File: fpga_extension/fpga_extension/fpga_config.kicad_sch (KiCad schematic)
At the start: 19 parts, among them U6 LFE5UM-85F-6BG381x

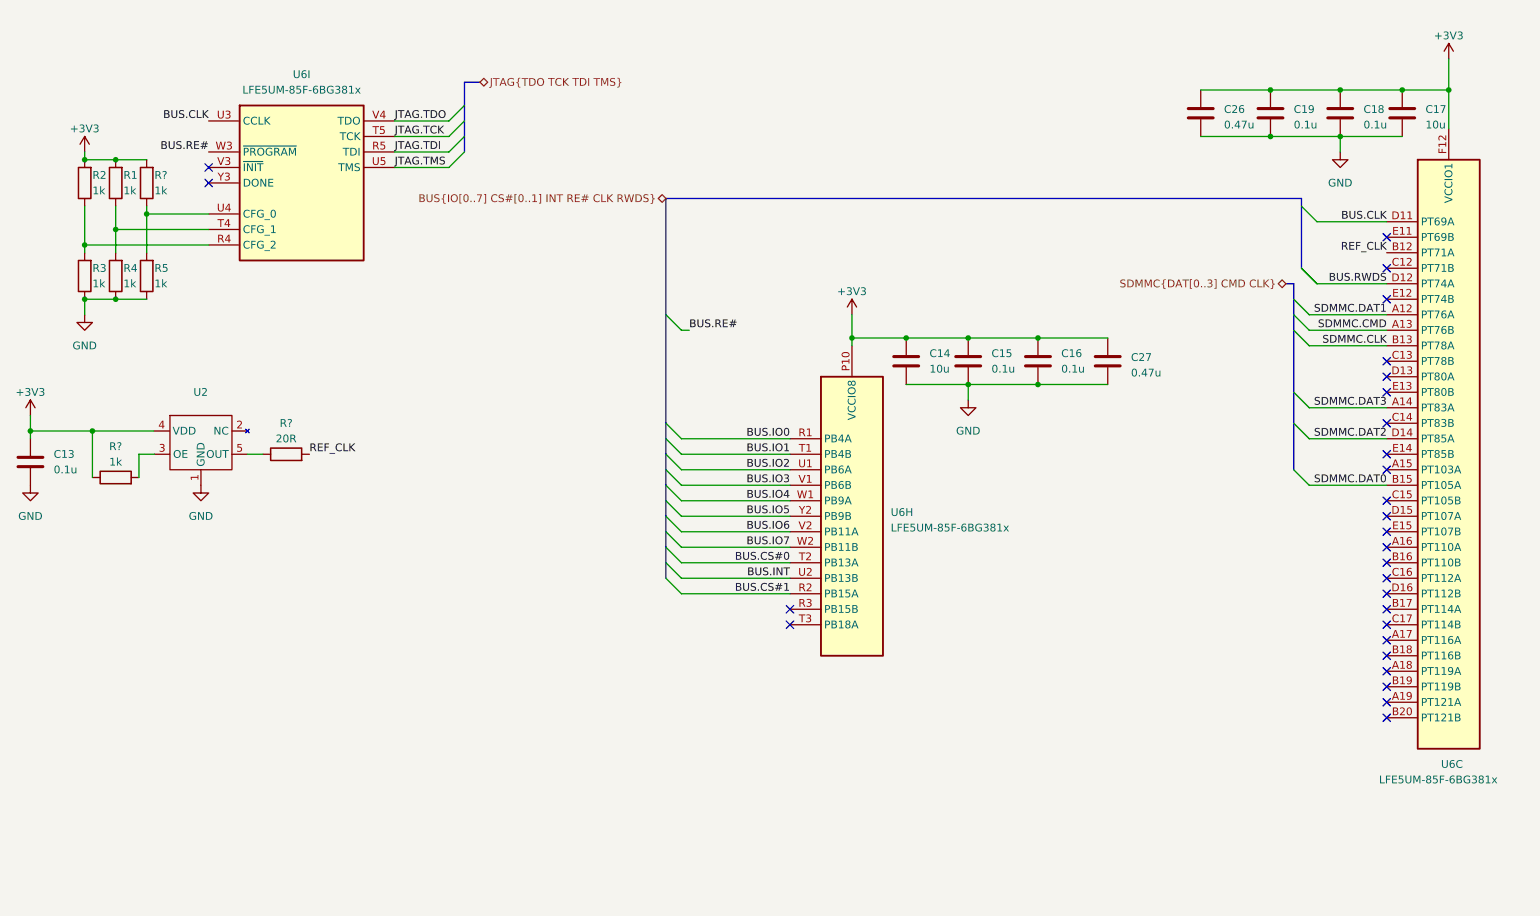
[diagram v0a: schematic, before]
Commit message: prepared first versions of PCBs
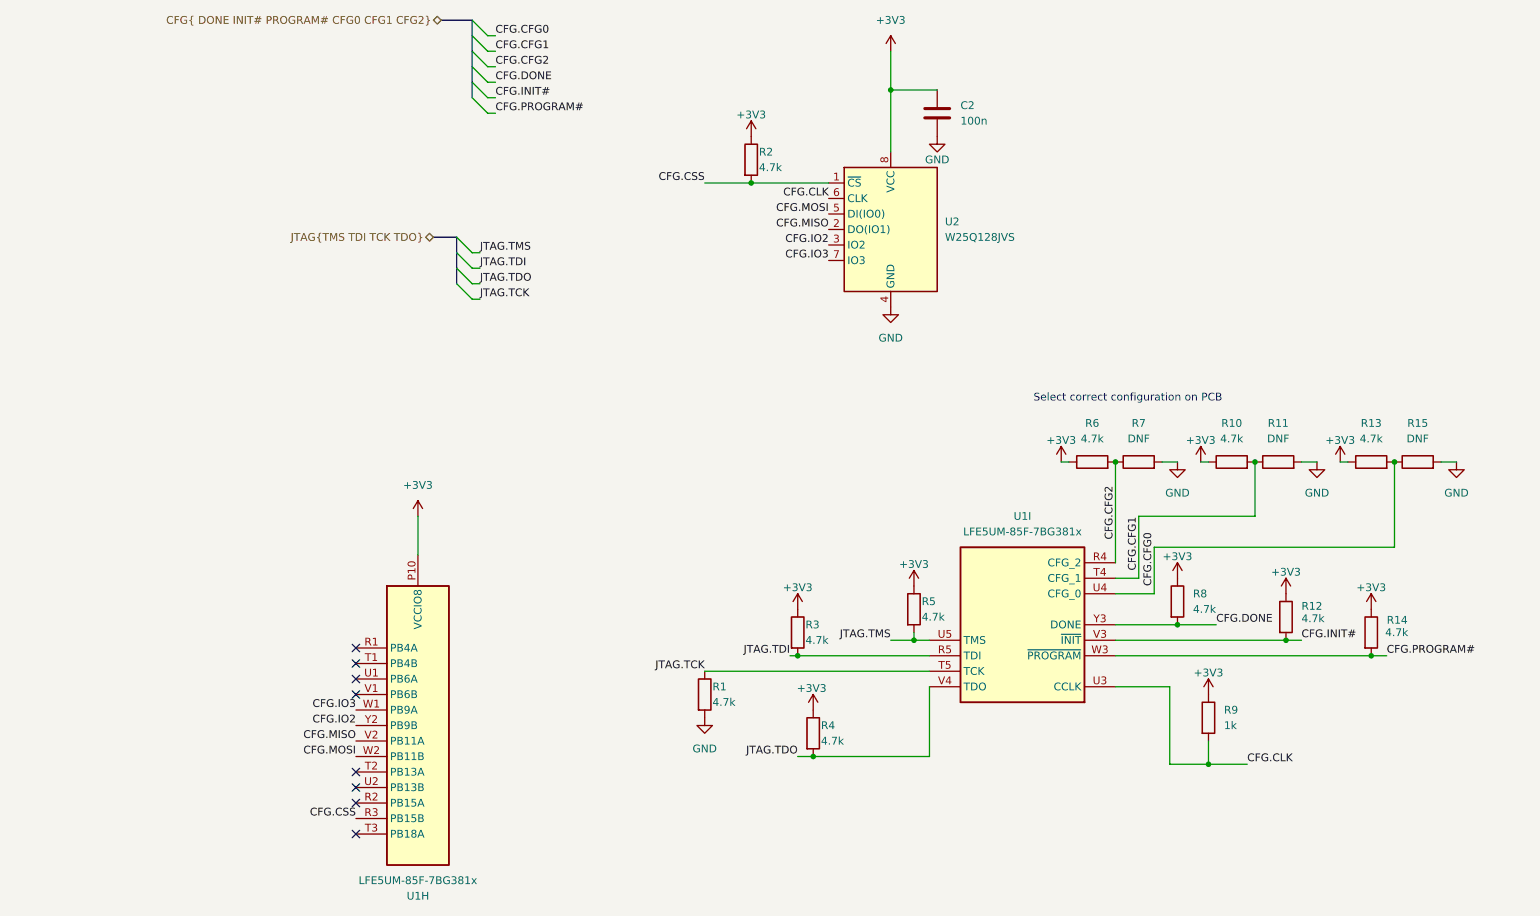
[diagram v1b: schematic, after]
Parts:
- removed C13, C15, C16, C18, C19: 0.1u, Capacitor_SMD:C_0201_0603Metric_Pad0.64x0.40mm_HandSolder, symbol Device:C
- removed C14, C17: 10u, Capacitor_SMD:C_0603_1608Metric_Pad1.08x0.95mm_HandSolder, symbol Device:C
- removed C26, C27: 0.47u, Capacitor_SMD:C_0201_0603Metric_Pad0.64x0.40mm_HandSolder, symbol Device:C
- removed R? (x2): 1k, symbol Device:R
- removed R?: 20R, symbol Device:R
- removed U2: ~, Package_TO_SOT_SMD:SOT-23-5, symbol fpga_extension_library:SiT2001B
- removed U6: LFE5UM-85F-6BG381x, Package_BGA:Lattice_caBGA-381_17.0x17.0mm_Layout20x20_P0.8mm_Ball0.4mm_Pad0.4mm_NSMD, symbol FPGA_Lattice:LFE5UM-85F-6BG381x
- added C2: 100n, Capacitor_SMD:C_0402_1005Metric_Pad0.74x0.62mm_HandSolder, symbol Device:C
- added R10, R12, R13, R14, R6, R8: 4.7k, Resistor_SMD:R_0402_1005Metric_Pad0.72x0.64mm_HandSolder, symbol Device:R
- added R11, R15, R7: DNF, Resistor_SMD:R_0402_1005Metric_Pad0.72x0.64mm_HandSolder, symbol Device:R
- added R9: 1k, Resistor_SMD:R_0402_1005Metric_Pad0.72x0.64mm_HandSolder, symbol Device:R
- added U1: LFE5UM-85F-7BG381x, Package_BGA:Lattice_caBGA-381_17.0x17.0mm_Layout20x20_P0.8mm_Ball0.4mm_Pad0.4mm_NSMD, symbol FPGA_Lattice:LFE5UM-85F-7BG381x
- added U2: W25Q128JVS, Package_SO:SOIC-8_5.23x5.23mm_P1.27mm, symbol Memory_Flash:W25Q128JVS
- R1, R2, R3, R4, R5: value 1k -> 4.7k; footprint (none) -> Resistor_SMD:R_0402_1005Metric_Pad0.72x0.64mm_HandSolder
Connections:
- net +3V3: now also R2.1, R3.1, R4.1, R5.1, C2.1, R10.1, R12.1, R13.1, R14.1, R6.1, R8.1, R9.1, U1.P10 (VCCIO8), U1.P9 (VCCIO8), U2.8 (VCC); no longer R1.2, R2.2
- net GND: now also R1.2, C2.2, R11.2, R15.2, R7.2, U2.4 (GND); no longer R3.1, R4.1, R5.1
- net JTAG.TCK: now also R1.1, U1.T5 (TCK)
- net JTAG.TDI: now also R3.2, U1.R5 (TDI)
- net JTAG.TDO: now also R4.2, U1.V4 (TDO)
- net JTAG.TMS: now also R5.2, U1.U5 (TMS)
- new net CFG.CFG0: R13.2, R15.1, U1.U4 (CFG_0)
- new net CFG.CFG1: R10.2, R11.1, U1.T4 (CFG_1)
- new net CFG.CFG2: R6.2, R7.1, U1.R4 (CFG_2)
- new net CFG.CLK: R9.2, U1.U3 (CCLK), U2.6 (CLK)
- new net CFG.CSS: R2.2, U1.R3 (PB15B), U2.1 (~{CS})
- new net CFG.DONE: R8.2, U1.Y3 (DONE)
- new net CFG.INIT#: R12.2, U1.V3 (~{INIT})
- new net CFG.IO2: U1.Y2 (PB9B), U2.3 (IO2)
- new net CFG.IO3: U1.W1 (PB9A), U2.7 (IO3)
- new net CFG.MISO: U1.V2 (PB11A), U2.2 (DO(IO1))
- new net CFG.MOSI: U1.W2 (PB11B), U2.5 (DI(IO0))
- new net CFG.PROGRAM#: R14.2, U1.W3 (~{PROGRAM})
- no-connect marks 28 -> 8
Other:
- note added: "Select correct configuration on PCB"
